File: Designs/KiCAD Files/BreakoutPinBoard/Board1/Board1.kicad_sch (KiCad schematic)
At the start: 7 parts, among them U1 STM32F405RGT7, U2 BME280, U3 BNO085, U4 H3LIS331DLTR, U5 MAX-M10S-00B, U6 FT232RL

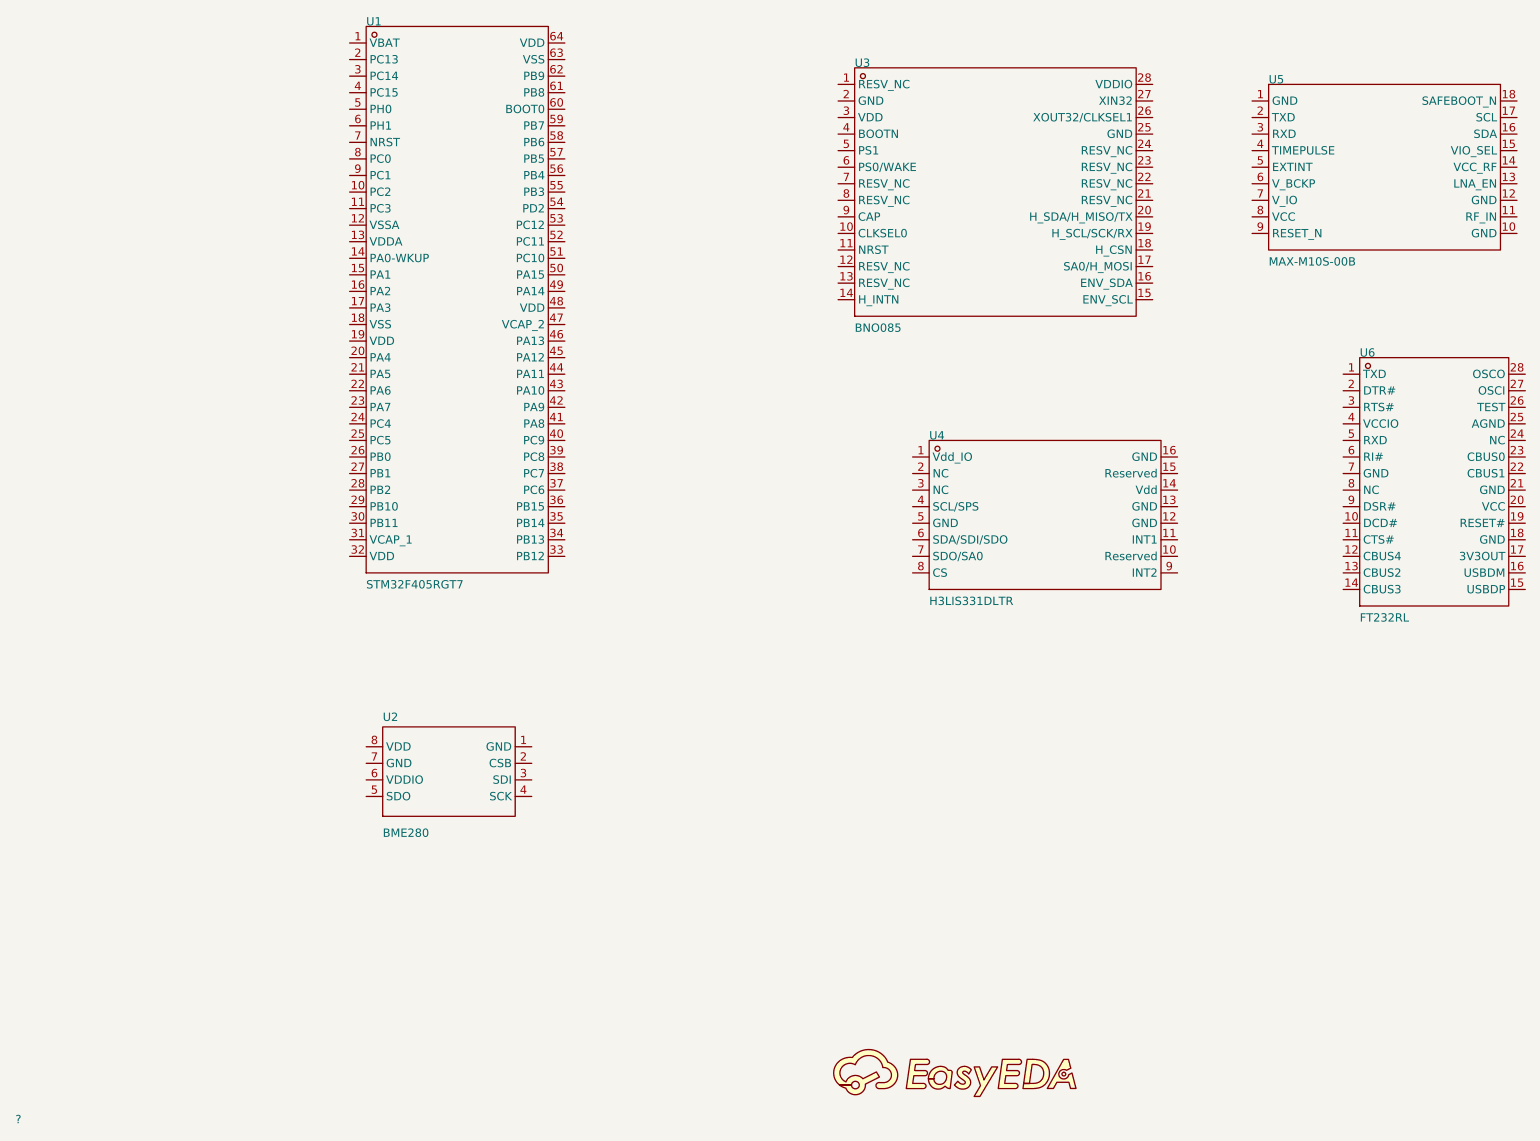
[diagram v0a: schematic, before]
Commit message: updating section
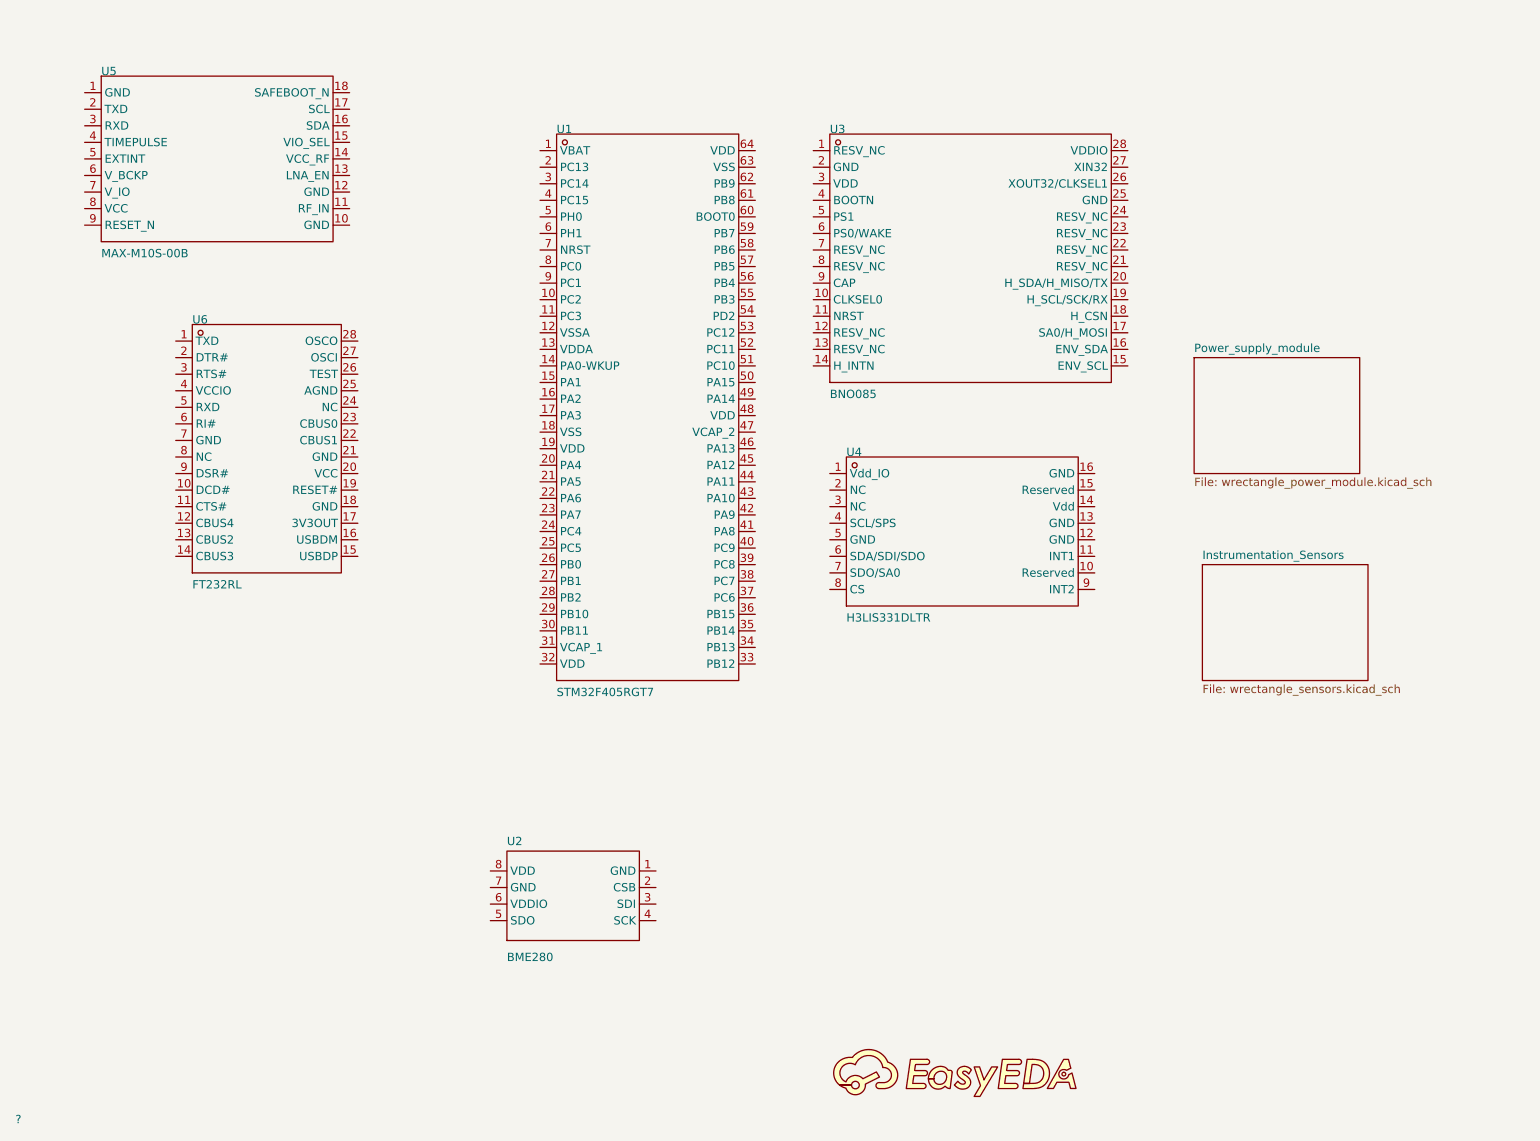
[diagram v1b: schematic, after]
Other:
- added sheet Instrumentation_Sensors (wrectangle_sensors.kicad_sch)
- added sheet Power_supply_module (wrectangle_power_module.kicad_sch)
- moved on the sheet: U1, U2, U3, U4, U5, U6
